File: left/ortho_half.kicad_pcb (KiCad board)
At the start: 2 copper layers, 150.9 x 146.1 mm, 60 parts, among them J1 AudioJack4, J2 Conn_01x01, J3 Conn_01x01, J4 Conn_01x01, J5 Conn_01x01, J6 Conn_01x01, J7 Conn_01x01, J8 Conn_01x01, J9 Conn_01x01, K11 KEYSW_RGB, K12 KEYSW_RGB, K13 KEYSW_RGB, K14 KEYSW_RGB, K15 KEYSW_RGB, K16 KEYSW_RGB, K21 KEYSW_RGB, K22 KEYSW_RGB, K23 KEYSW_RGB, K24 KEYSW_RGB, K25 KEYSW_RGB, K26 KEYSW_RGB, K31 KEYSW_RGB, K32 KEYSW_RGB, K33 KEYSW_RGB, K34 KEYSW_RGB, K35 KEYSW_RGB, K36 KEYSW_RGB, K41 KEYSW_RGB, K42 KEYSW_RGB, K43 KEYSW_RGB, K44 KEYSW_RGB, K45 KEYSW_RGB, K46 KEYSW_RGB, K51 KEYSW_RGB, K52 KEYSW_RGB, K53 KEYSW_RGB, K54 KEYSW_RGB, K55 KEYSW_RGB, K56 KEYSW_RGB, K61 KEYSW_RGB, K62 KEYSW_RGB, K63 KEYSW_RGB, K64 KEYSW_RGB, K65 KEYSW_RGB, K66 KEYSW_RGB, SW1 SW_PUSH_RESET, U1 EliteC, U2 IS31FL3733-TQ

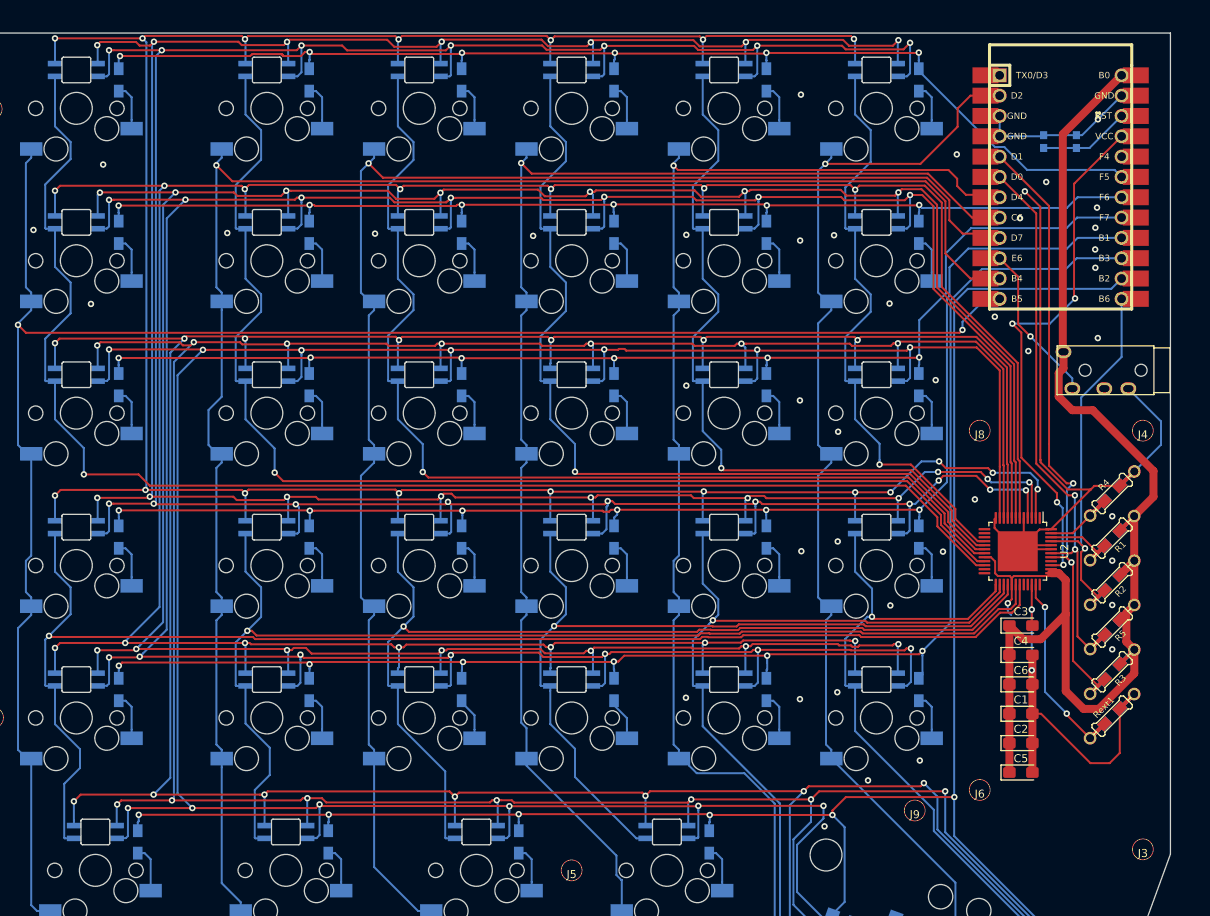
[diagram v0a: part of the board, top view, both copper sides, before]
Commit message: Some initial work on the PCB update.
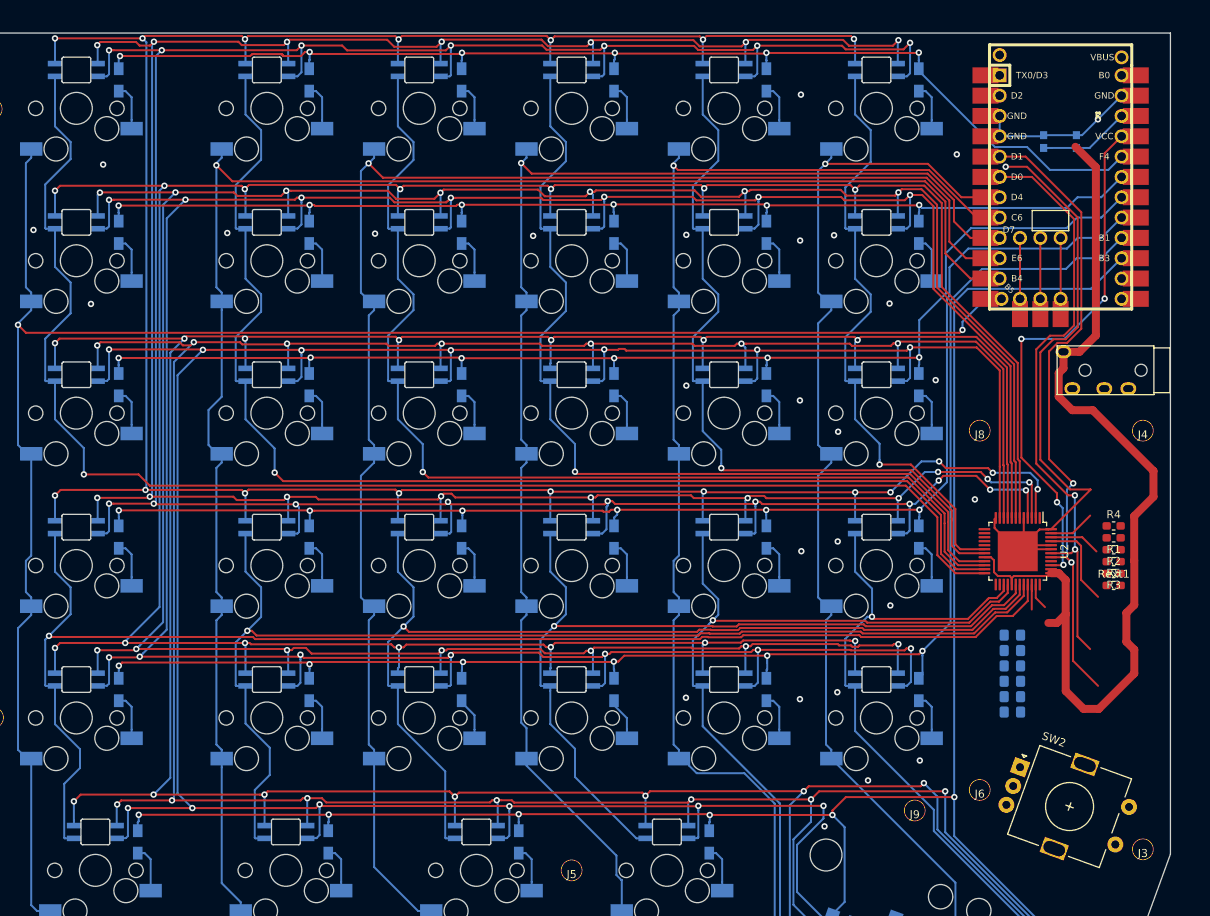
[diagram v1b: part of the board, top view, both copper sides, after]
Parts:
- added SW2: Rotary_Encoder_Switch, Keebio-Parts:RotaryEncoder_Alps_EC11E-Switch_Vertical_H20mm, F.Cu at (143.2, 111.1)
- C1, C2, C3, C4, C5, C6: footprint Capacitor_Tantalum_SMD:CP_EIA-3216-10_Kemet-I_Pad1.58x1.35mm_HandSolder -> Capacitor_SMD:C_0805_2012Metric_Pad1.15x1.40mm_HandSolder; moved to B.Cu
- R1, R2, R3, R4, R5, Rext1: footprint Keebio-Parts:Resistor-Hybrid -> Resistor_SMD:R_0603_1608Metric_Pad1.05x0.95mm_HandSolder
- U1: value EliteC -> microctrl_superset; footprint Keebio-Parts:Elite-C-castellated-24pin-holes -> vladkvit_keyb:microcontroller_eliteC_ninenano
- moved C5 17.2 mm to (136.1, 89.7)
- moved Rext1 16.3 mm to (148.7, 83.5), turned to 0 degrees
- moved R3 12.3 mm to (148.7, 82.0), turned to 180 degrees
- moved C2 11.6 mm to (136.1, 91.6)
- moved C3 10.9 mm to (136.1, 99.3)
- moved R5 8.17 mm to (148.7, 80.5), turned to 180 degrees
- moved C1 6.07 mm to (136.1, 93.5)
- moved R2 4.13 mm to (148.7, 79.0), turned to 180 degrees
- moved R4 4.06 mm to (148.7, 76.0), turned to 0 degrees
- moved C4 3.46 mm to (136.1, 95.4)
- moved C6 1.87 mm to (136.1, 97.4)
- moved R1 0.20 mm to (148.7, 77.5), turned to 180 degrees
- turned U1 to 0 degrees
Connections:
- R1 pad 1: VCC -> VIO
- U1 pad 1: col7 -> col8
- U1 pad 10: serial -> col3
- U1 pad 13: INTB -> Net-(U1-Pad13)
- U1 pad 14: row6 -> serial
- U1 pad 15: row5 -> row6
- U1 pad 16: row4 -> row5
- U1 pad 17: row3 -> row4
- U1 pad 18: row2 -> row3
- U1 pad 19: row1 -> row2
- U1 pad 2: col6 -> col7
- U1 pad 20: Net-(U1-Pad20) -> row1
- U1 pad 24: VCC -> Net-(SW3-Pad2)
- U1 pad 7: col5 -> col6
- U1 pad 8: col4 -> col5
- U1 pad 9: col3 -> col4
- U2 pad 16: led_col6 -> (no net)
- U2 pad 17: led_col5 -> (no net)
- U2 pad 18: led_col4 -> led_col6
- U2 pad 19: led_col3 -> led_col5
- U2 pad 21: led_col2 -> led_col4
- U2 pad 22: led_col1 -> led_col3
- U2 pad 23: (no net) -> led_col2
- U2 pad 24: (no net) -> led_col1
- U2 pad 25: led_col14 -> (no net)
- U2 pad 26: led_col13 -> (no net)
- U2 pad 27: led_col12 -> led_col14
- U2 pad 28: led_col11 -> led_col13
- U2 pad 30: led_col10 -> led_col12
- U2 pad 31: led_col9 -> led_col11
- U2 pad 32: (no net) -> led_col10
- U2 pad 33: (no net) -> led_col9
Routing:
- net GND: track 161.7 -> 110.8 mm, vias 45 -> 29
- net VCC: track 160.5 -> 119.6 mm, vias 1 -> 0
- net INTB: track 47.0 -> 11.2 mm, vias 1 -> 0
- net serial: track 21.8 -> 1.78 mm, vias 1 -> 0
- net Net-(Rext1-Pad1): track 22.0 -> 3.30 mm, vias 2 -> 0
- net encA2: track 0.00 -> 9.52 mm
- net encA1: track 0.00 -> 9.52 mm
- net Net-(U1-Pad27): track 0.00 -> 9.52 mm
- net SCL: track 69.2 -> 76.5 mm
- net SDA: track 77.0 -> 82.4 mm
- net col6: track 141.8 -> 138.7 mm
- net led_col4: track 113.2 -> 115.9 mm
- net led_col3: track 132.5 -> 135.2 mm
- net col4: track 165.0 -> 167.6 mm
- net col3: track 187.9 -> 190.5 mm
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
